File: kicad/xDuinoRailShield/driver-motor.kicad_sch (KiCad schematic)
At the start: 6 parts, among them U801 BDR6133, U802 DRV8872DDAR_SOP-8-EP

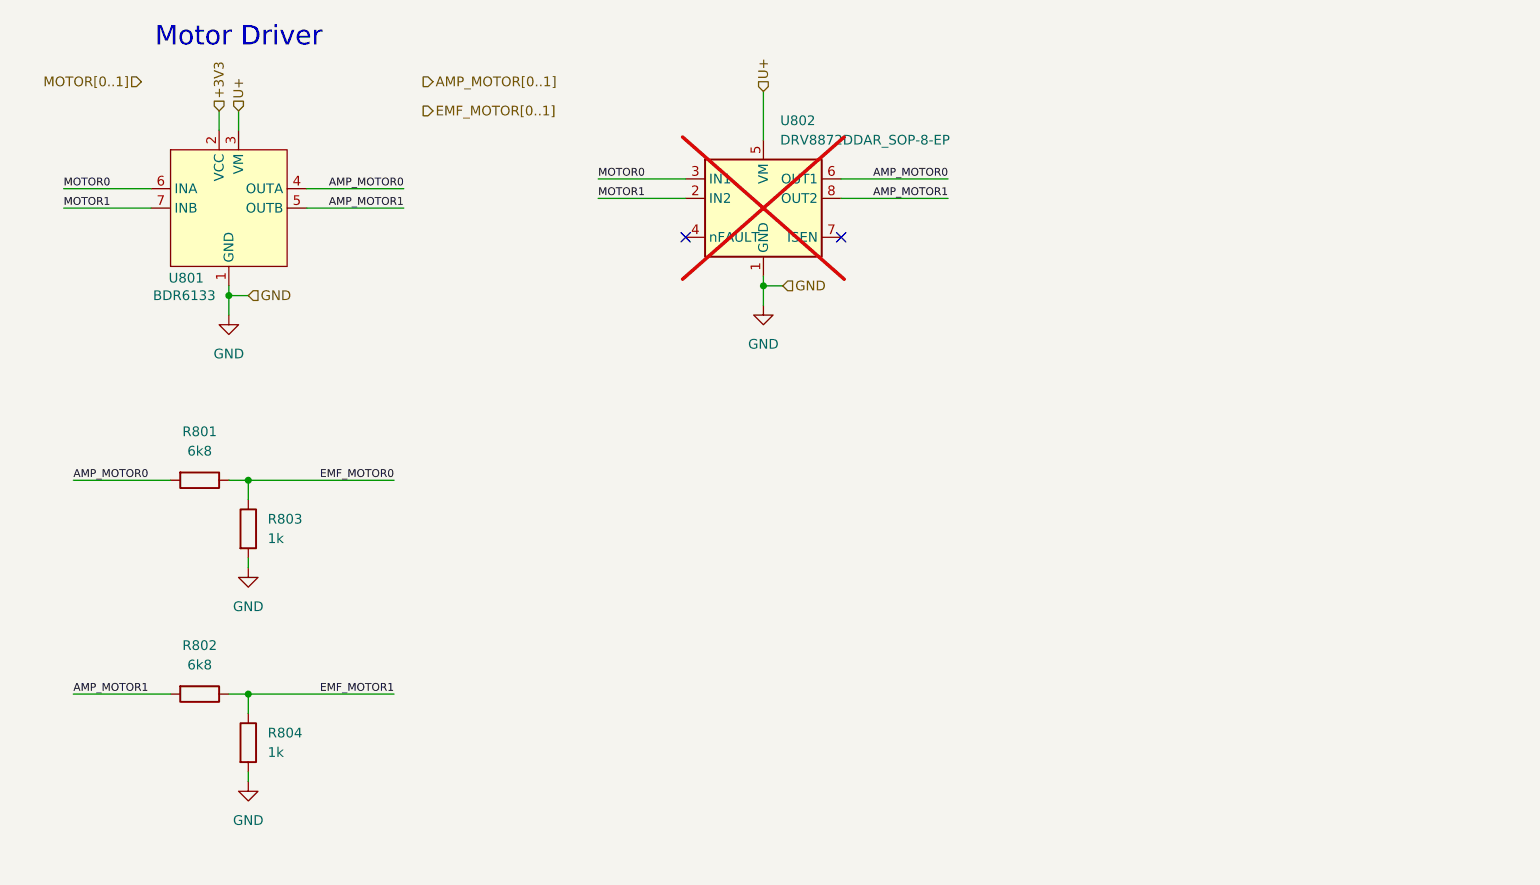
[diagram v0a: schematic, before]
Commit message: Many exiting news
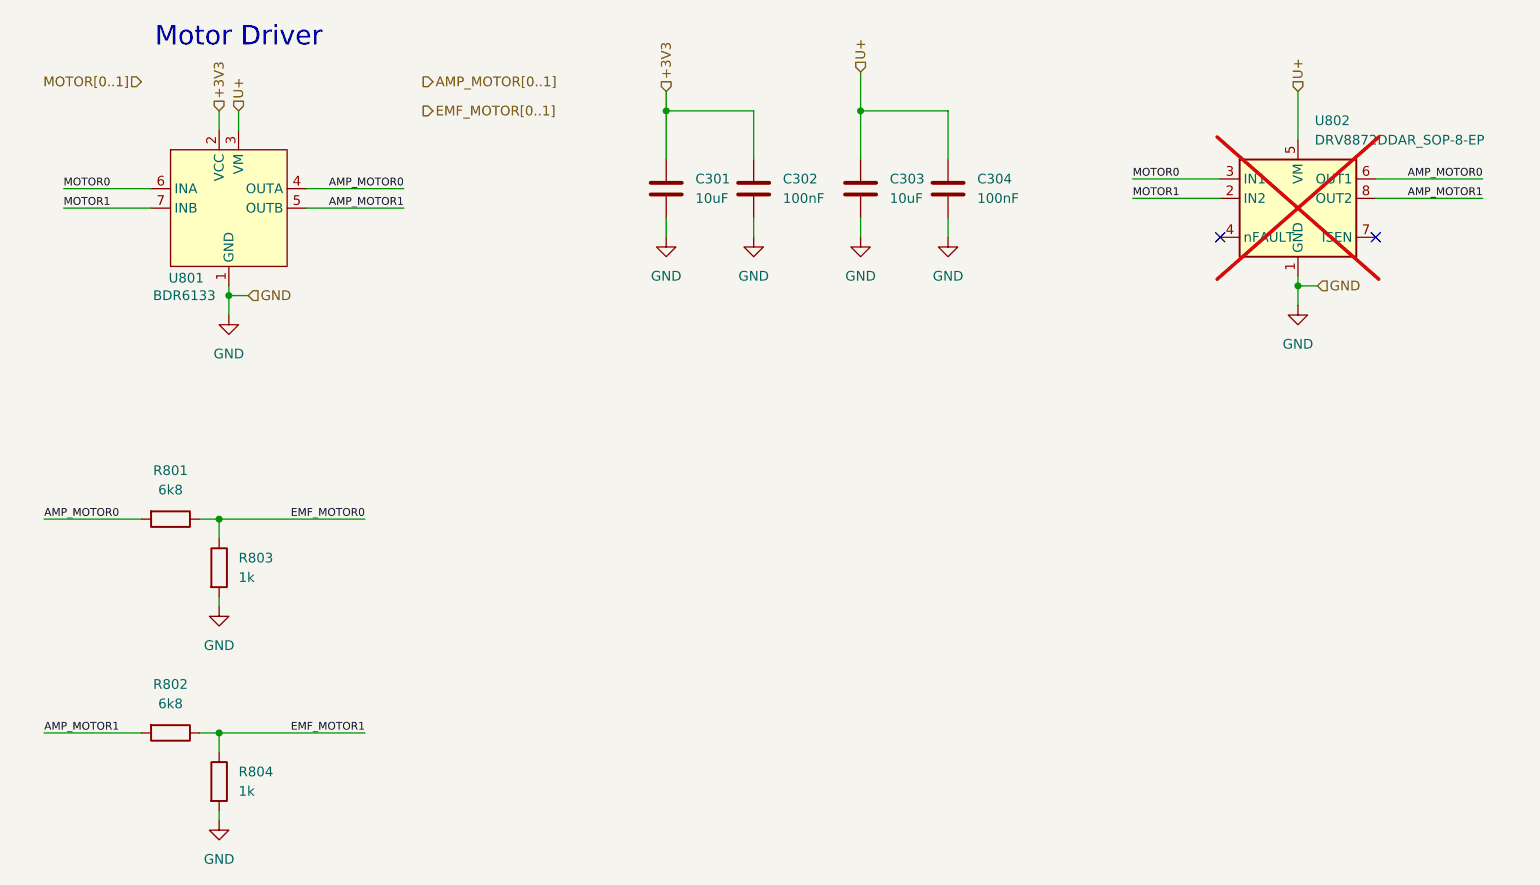
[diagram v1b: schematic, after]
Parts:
- added C301, C303: 10uF, Capacitor_SMD:C_0805_2012Metric_Pad1.18x1.45mm_HandSolder, symbol Device:C
- added C302, C304: 100nF, Capacitor_SMD:C_0805_2012Metric_Pad1.18x1.45mm_HandSolder, symbol Device:C
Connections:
- net +3V3: now also C301.1, C302.1
- net GND: now also C301.2, C302.2, C303.2, C304.2
- net U+: now also C303.1, C304.1
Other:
- moved on the sheet: R801, R802, R803, R804, U802
